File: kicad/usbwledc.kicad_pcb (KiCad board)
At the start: 4 copper layers, 40 x 35 mm, 31 parts, among them J1 5V PAD, J10 USB_C_Receptacle_USB2.0, J2 D1 PAD, J3 GND PAD, J4 5V PAD, J5 D2 PAD, J6 GND PAD, J7 Conn_01x04_Pin, SW1 FLASH_SW, U1 CH340N, U2 AMS1117-3.3, U3 ESP32-WROOM-32

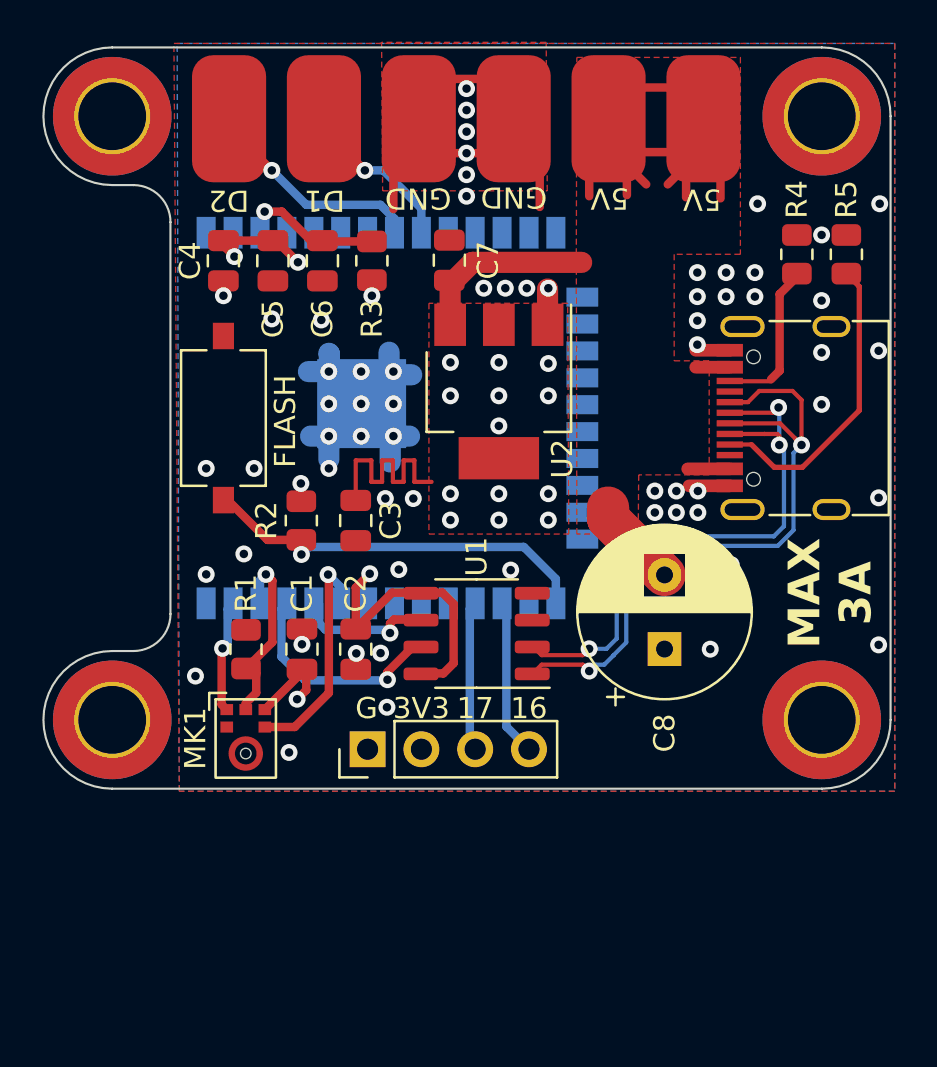
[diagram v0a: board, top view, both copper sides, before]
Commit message: v1.1
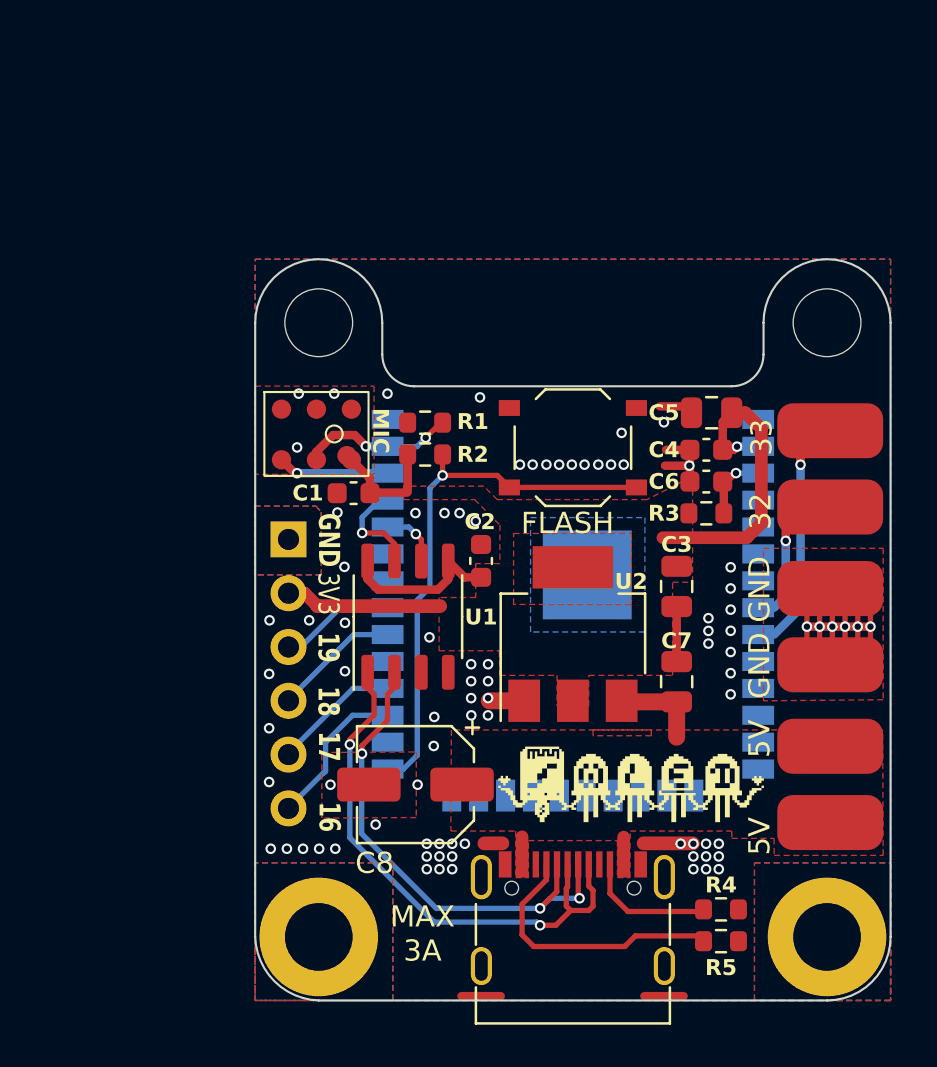
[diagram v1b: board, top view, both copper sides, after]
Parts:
- C1, C2, C4, C6: footprint Capacitor_SMD:C_0805_2012Metric -> Capacitor_SMD:C_0603_1608Metric
- C3, C7: value 22uF -> 10uF
- C8: value 330uF -> 100uF; footprint Capacitor_THT:CP_Radial_D8.0mm_P3.50mm -> Capacitor_SMD:CP_Elec_5x5.4
- G***: moved to F.Cu
- H1, H2, H3, H4: footprint MountingHole:MountingHole_3.2mm_M3_DIN965_Pad_TopBottom -> MountingHole:MountingHole_3.2mm_M3_DIN965_Pad
- J1, J2, J3, J4, J5, J6: footprint ProjectLibrary:SolderWirePad_1x01_SMD_3x6mm -> Library:SolderWirePad_1x01_SMD_3x6mm
- J7: value Conn_01x04_Pin -> Accessories; footprint Connector_PinHeader_2.54mm:PinHeader_1x04_P2.54mm_Vertical -> Connector_PinHeader_2.54mm:PinHeader_1x06_P2.54mm_Vertical
- MK1: value ICS-43434 -> GSA4737; footprint Sensor_Audio:InvenSense_ICS-43434-6_3.5x2.65mm -> microphone:Microphone-6pin
- R1, R2, R3, R4, R5: footprint Resistor_SMD:R_0805_2012Metric -> Resistor_SMD:R_0603_1608Metric
- SW1: footprint Button_Switch_SMD:SW_Tactile_SPST_NO_Straight_CK_PTS636Sx25SMTRLFS -> Button_Switch_SMD:SW_Push_1P1T_XKB_TS-1187A
- moved H1 40.0 mm to (33.0, 62.0)
- moved H2 38.8 mm to (57.0, 62.0)
- moved G*** 35.1 mm to (47.8, 54.8), turned to 0 degrees
- moved J1 33.8 mm to (57.1, 56.6), turned to 90 degrees
- moved R5 33.0 mm to (52.0, 62.2), turned to 0 degrees
- moved J5 32.0 mm to (57.1, 38.1), turned to 90 degrees
- moved J4 31.4 mm to (57.1, 53.0), turned to 90 degrees
- moved R4 31.1 mm to (52.0, 60.7), turned to 0 degrees
- moved J2 30.1 mm to (57.1, 41.7), turned to 90 degrees
- moved J3 29.8 mm to (57.1, 49.1), turned to 90 degrees
- moved J6 29.5 mm to (57.1, 45.5), turned to 90 degrees
- moved J10 27.2 mm to (45.0, 62.3), turned to 0 degrees
- moved C4 24.5 mm to (51.3, 39.0), turned to 0 degrees
- moved C7 22.6 mm to (49.9, 50.0)
- moved C5 21.9 mm to (51.5, 37.2), turned to 180 degrees
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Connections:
- C8 pad 1: GND -> +5V
- C8 pad 2: +5V -> GND
- J10 pad S1: unconnected-(J10-SHIELD-PadS1) -> GND
- J7 pad 3: IO17 -> IO19
- J7 pad 4: IO16 -> IO18
- MK1 pad 1: I2S_WS -> GND
- MK1 pad 2: GND -> unconnected-(MK1-WS-Pad2)
- MK1 pad 5: +3V3 -> I2S_SD
- MK1 pad 6: I2S_SD -> +3V3
- U3 pad 30: unconnected-(U3-IO18-Pad30) -> IO18
- U3 pad 31: unconnected-(U3-IO19-Pad31) -> IO19
- U3 pad 33: I2S_SCK -> unconnected-(U3-IO21-Pad33)
- U3 pad 36: I2S_SD -> I2S_SCK
- U3 pad 37: I2S_WS -> I2S_SD
- U3 pad 8: STRIP_DATA_2 -> STRIP_DATA_1
- U3 pad 9: STRIP_DATA_1 -> STRIP_DATA_2
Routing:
- net +5V: track 32.9 -> 6.52 mm
- net FLASH: track 18.9 -> 25.8 mm
- net IO18: track 0.00 -> 6.06 mm
- net I2S_SCK: track 10.9 -> 5.27 mm
- net IO19: track 0.00 -> 5.53 mm
- net I2S_WS: track 5.34 -> 0.00 mm, vias 1 -> 0
- net TX: track 10.2 -> 4.83 mm
- net D+: track 31.6 -> 26.3 mm
- net RX: track 6.50 -> 2.86 mm
- net D-: track 27.8 -> 24.2 mm
- net GND: track 23.6 -> 27.0 mm, vias 64 -> 85
- net Net-(U3-EN): track 6.37 -> 3.14 mm
- net STRIP_DATA_1: track 7.29 -> 4.63 mm
- net Net-(J10-CC1): track 14.4 -> 12.9 mm
- net I2S_SD: track 8.56 -> 7.36 mm, vias 1 -> 2
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- removed copper zone on In2.Cu, net +3V3
- removed copper zone on In1.Cu, net GND
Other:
- board size 40 x 35 mm -> 30 x 35 mm
- copper layers 4 -> 2
- board text added: "18"
- board text added: "19"
- board text added: "22"
- board text added: "23"
- board text added: "32"
- board text added: "33"
- board text added: "MIC"
- board text added: "NANDXOR"
- board text added: "SD"
- board text added: "WS"
- board text added: "v1.1"
- board text removed: "D1"
- board text removed: "D2"
- board text removed: "G"
- board text removed: "JLCJLCJLC"
- board text removed: "NANDXOR's"
- board text removed: "v1.0"
